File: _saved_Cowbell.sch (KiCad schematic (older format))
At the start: 23 parts, among them J1 Conn_Coaxial, J102 Conn_01x02_Male, J104 Conn_01x02_Male, J105 Conn_01x02_Male, J401 Conn_Coaxial, Q102 DMG6601LVT, U101 SIM28ML, U102 LSM303C, U103 ESP32-WROOM-32, U105 RFM9x

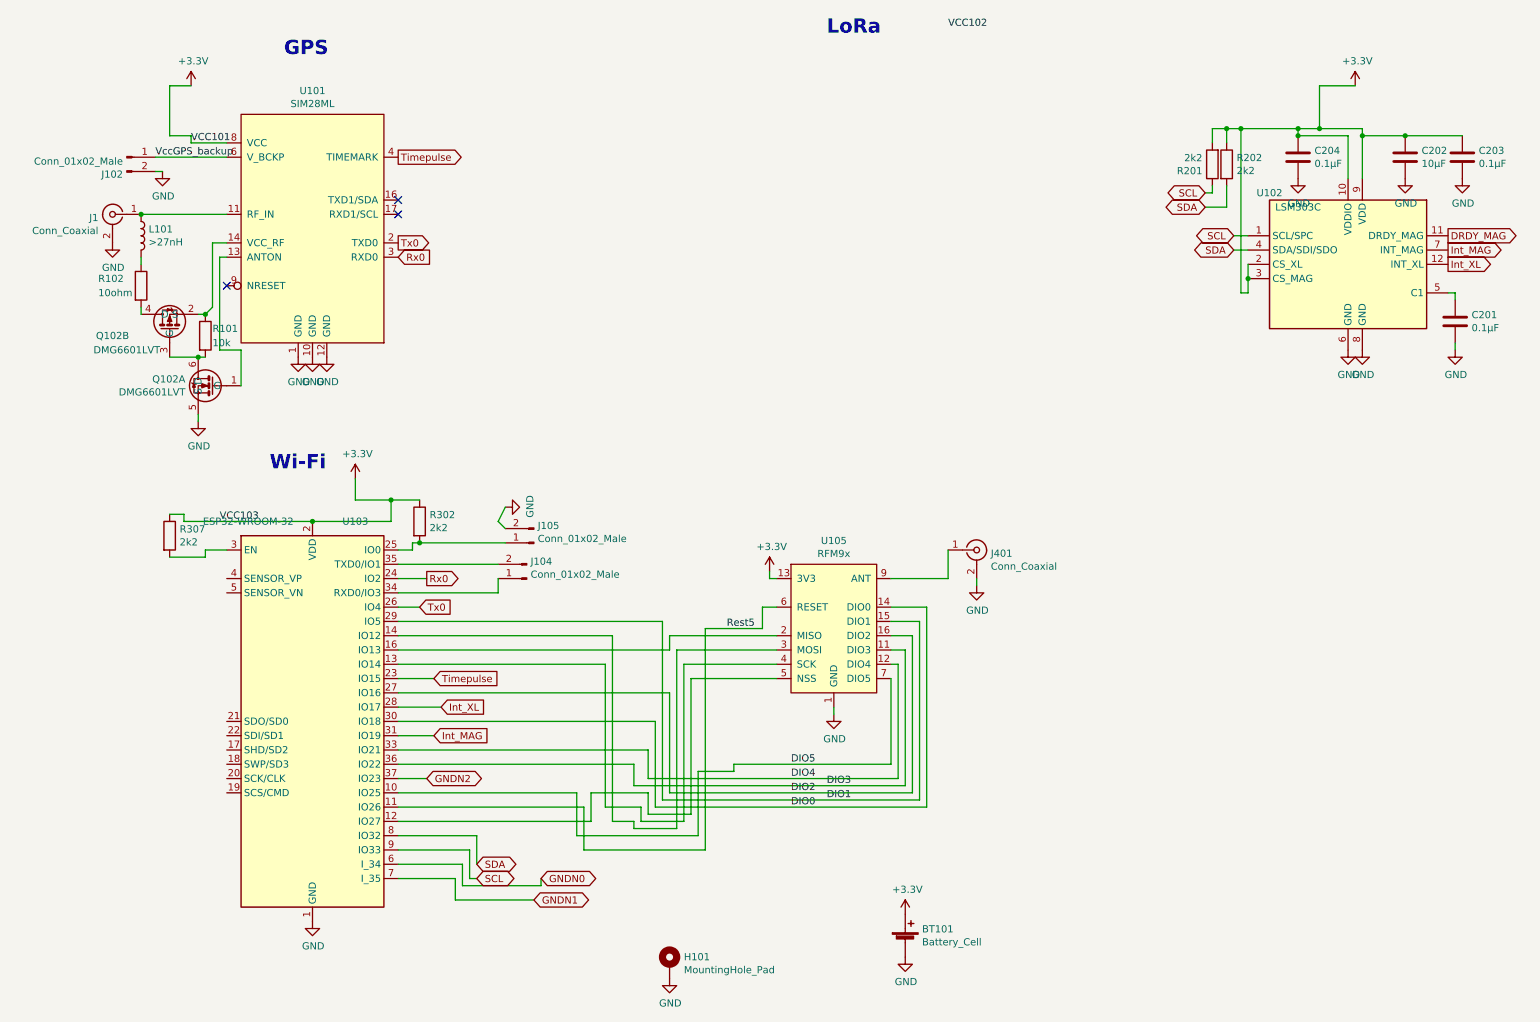
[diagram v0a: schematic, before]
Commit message: Updated to newest version
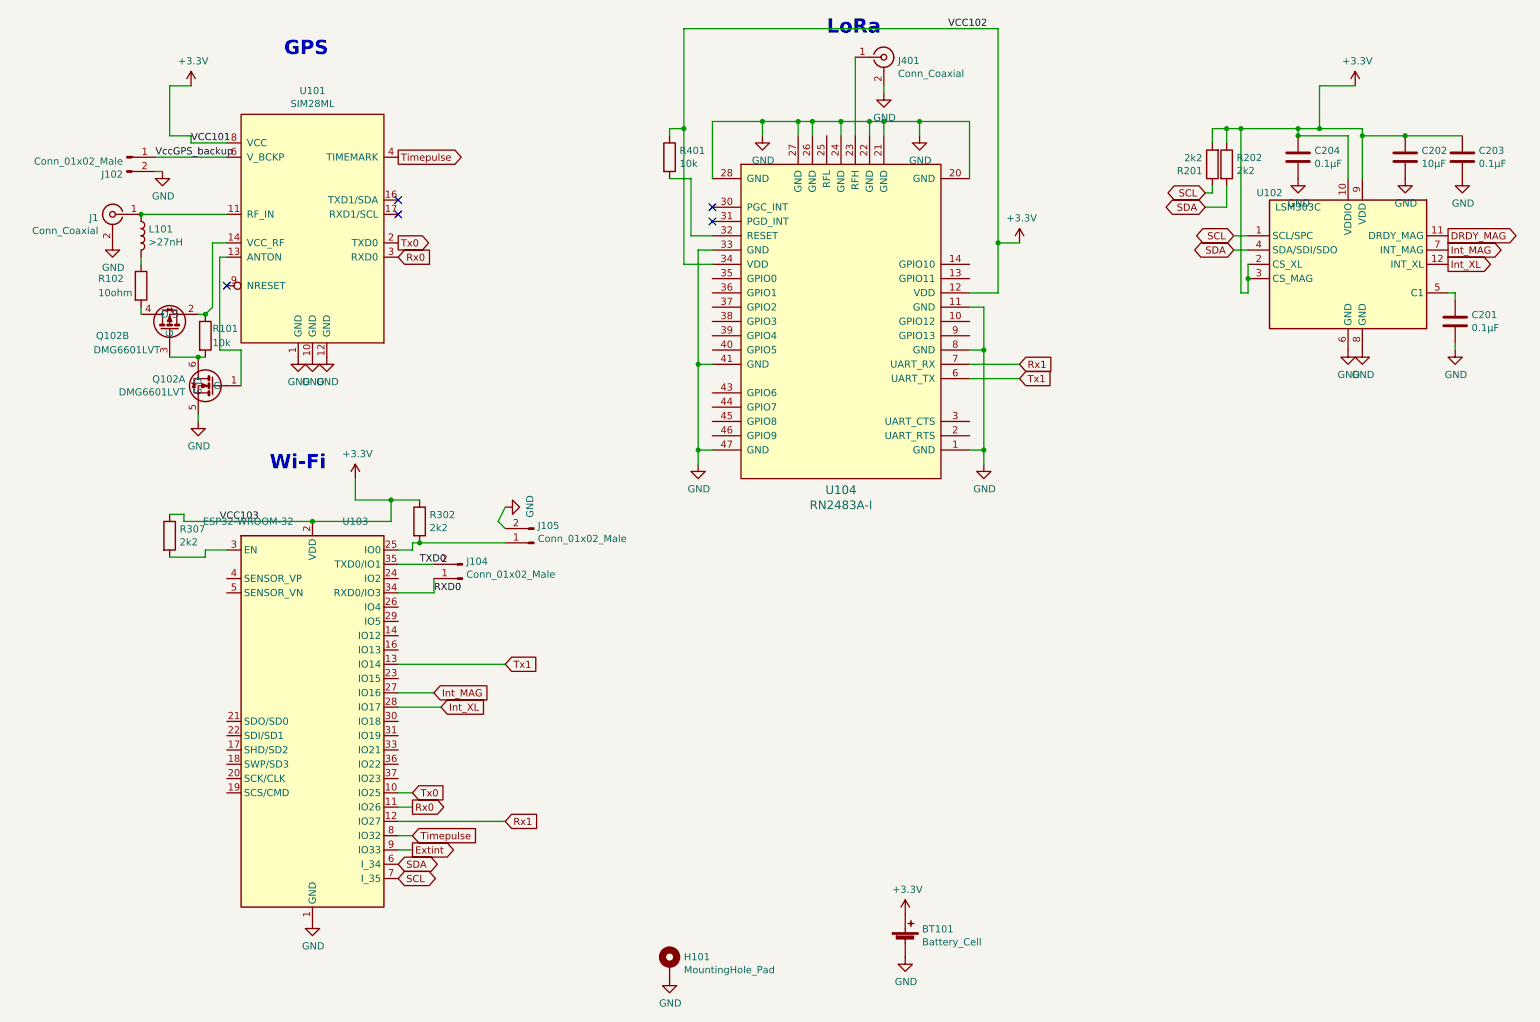
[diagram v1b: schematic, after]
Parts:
- removed U105: RFM9x, Emborg:RFM95, symbol Emborg:RFM9x
- added R401: 10k, Resistor_SMD:R_0603_1608Metric, symbol Device:R
- added U104: RN2483A-I, Emborg:RN2483, symbol Emborg:RN2483A-I
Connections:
- net DIO2 is gone; now on net Int_MAG: U103.27 (IO16)
- net DIO5 is gone; now on net Tx0: U103.10 (IO25)
- net GNDN0 is gone; now on net SDA: U103.6 (I_34)
- net GNDN1 is gone; now on net SCL: U103.7 (I_35)
- net Rest5 is gone; now on net Rx0: U103.11 (IO26)
- net +3V3: now also R401.1, U104.12 (VDD), U104.34 (VDD)
- net GND: now also U104.1 (GND), U104.11 (GND), U104.20 (GND), U104.21 (GND), U104.22 (GND), U104.24 (GND), U104.26 (GND), U104.27 (GND), U104.28 (GND), U104.33 (GND), U104.41 (GND), U104.47 (GND), U104.8 (GND)
- net Int_MAG: no longer U103.31 (IO19)
- net Rx0: no longer U103.24 (IO2)
- net SCL: no longer U103.9 (IO33)
- net SDA: no longer U103.8 (IO32)
- net Timepulse: now also U103.8 (IO32); no longer U103.23 (IO15)
- net Tx0: no longer U103.26 (IO4)
- net Rx1: now reaches U103.12 (IO27)
- net Rx1: now also U104.7 (UART_RX)
- net Tx1: now reaches U103.13 (IO14)
- net Tx1: now also U104.6 (UART_TX)
- net RXD0: now reaches J104.1 (Pin_1), U103.34 (RXD0/IO3)
- net TXD0: now reaches J104.2 (Pin_2), U103.35 (TXD0/IO1)
- net at J401.1 (In): now also U104.23 (RFH)
- net DIO0: no longer names the net of U103.30 (IO18)
- net DIO1: no longer names the net of U103.29 (IO5)
- net DIO3: no longer names the net of U103.36 (IO22)
- net DIO4: no longer names the net of U103.33 (IO21)
- net GNDN2: no longer names the net of U103.37 (IO23)
- new net: R401.2, U104.32 (RESET)
- new net Extint: U103.9 (IO33)
- no-connect marks 3 -> 5
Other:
- moved on the sheet: J104, J401
